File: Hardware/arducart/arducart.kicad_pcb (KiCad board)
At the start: 2 copper layers, 53 x 36.2 mm, 11 parts, among them J2 AVR-ISP-6

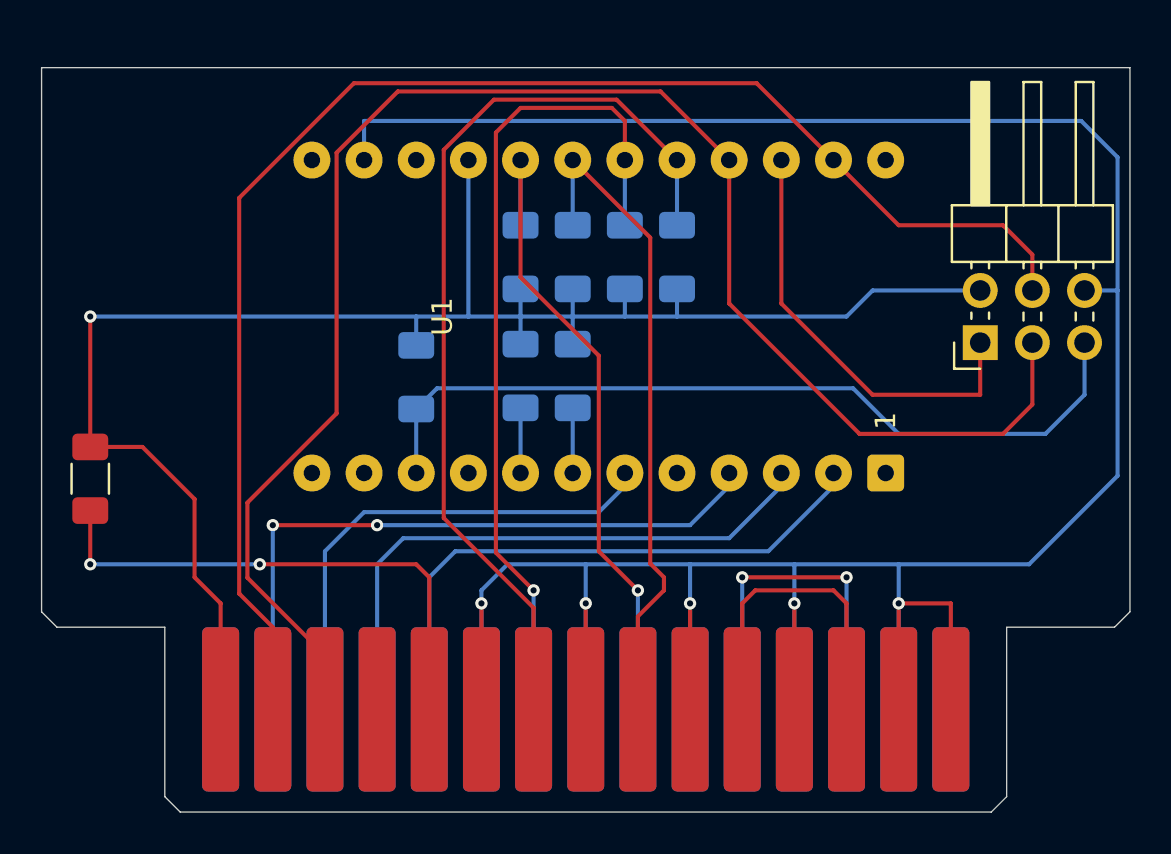
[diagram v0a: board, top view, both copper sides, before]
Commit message: Finish PCB design
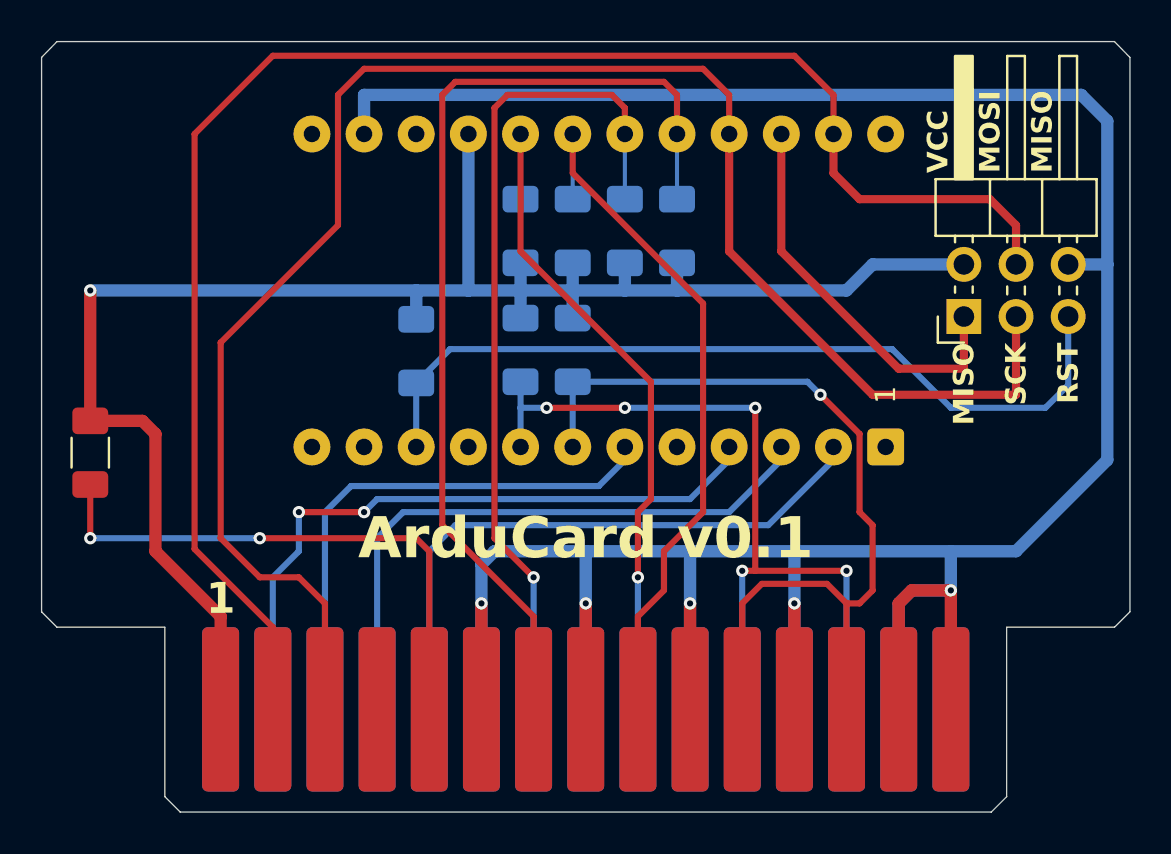
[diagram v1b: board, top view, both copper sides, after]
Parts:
- moved J2 1.50 mm to (160.9, 80.9)
- moved R2 1.27 mm to (141.9, 82.5)
- moved R3 1.27 mm to (146.9, 76.7)
- moved R4 1.27 mm to (144.4, 76.7)
- moved R5 1.27 mm to (141.9, 76.7)
- moved R6 1.27 mm to (139.3, 76.7)
- moved R8 1.27 mm to (134.2, 82.6)
- moved U1 1.27 mm to (141.9, 79.6)
- moved R1 1.27 mm to (118.4, 87.5)
- moved R7 1.27 mm to (139.3, 82.5)
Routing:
- net BTN_A: track 19.1 -> 43.8 mm, vias 0 -> 1
- net BTN_B: track 21.1 -> 41.1 mm, vias 2 -> 5
- net ISP_MOSI: track 71.7 -> 78.7 mm
- net GND: track 157.3 -> 164.1 mm
- net ISP_SCK: track 80.4 -> 83.9 mm
- net BTN_UP: track 45.8 -> 48.8 mm
- net BTN_LEFT: track 32.3 -> 35.1 mm
- net SCREEN_RESET: track 23.6 -> 25.9 mm
- net SCREEN_DC: track 28.3 -> 30.2 mm
- net BTN_RIGHT: track 32.3 -> 34.1 mm
- net ISP_MISO: track 21.1 -> 19.5 mm
- net Net-(J1-BTN_MENU1): track 25.8 -> 27.1 mm
- net BUZZER: track 28.0 -> 29.2 mm
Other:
- board size 53 x 36.2 mm -> 53 x 37.5 mm
- board text added: "1"
- board text added: "30"
- board text added: "ArduCard v0.1"
- board text added: "MISO"
- board text added: "MOSI"
- board text added: "RST"
- board text added: "SCK"
- board text added: "VCC"
